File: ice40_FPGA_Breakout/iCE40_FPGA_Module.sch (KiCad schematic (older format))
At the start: 104 parts, among them U1 iCE40HX8_CT256

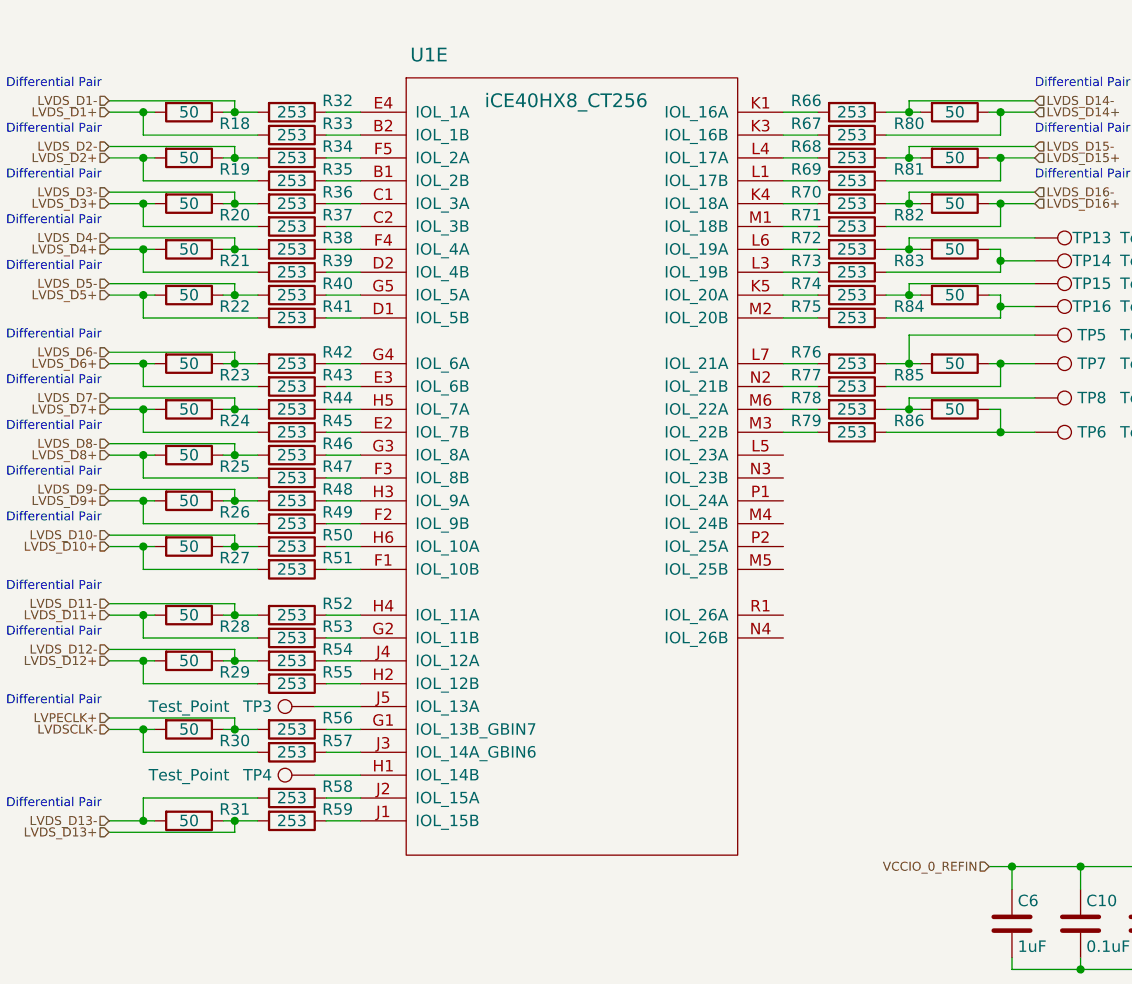
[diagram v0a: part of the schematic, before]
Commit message: Regrouping con't
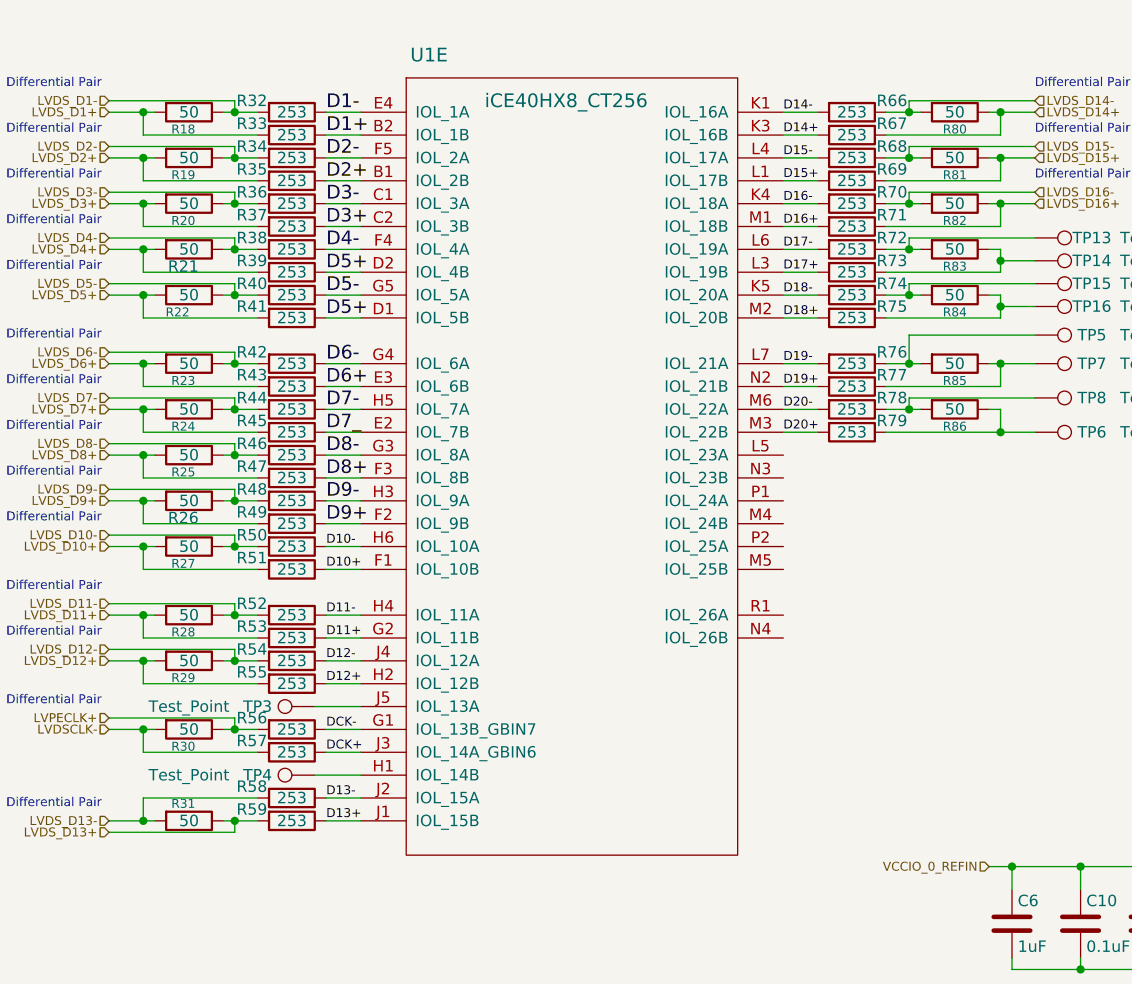
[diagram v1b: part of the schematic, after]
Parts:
- TP1: footprint TestPoint:TestPoint_Plated_Hole_D2.0mm -> TestPoint:TestPoint_THTPad_D1.0mm_Drill0.5mm
- TP2, TP3, TP4: footprint TestPoint:TestPoint_Pad_D2.0mm -> TestPoint:TestPoint_THTPad_D1.0mm_Drill0.5mm
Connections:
- net D2+: now reaches R35.1, U1.B1 (IOL_2B)
- net D1+: now reaches R33.1, U1.B2 (IOL_1B)
- net D3-: now reaches R36.1, U1.C1 (IOL_3A)
- net D3+: now reaches R37.1, U1.C2 (IOL_3B)
- net D5+: now reaches R41.1, U1.D1 (IOL_5B)
- net D5+: now also R39.1, U1.D2 (IOL_4B)
- net D7_: now reaches R45.1, U1.E2 (IOL_7B)
- net D6+: now reaches R43.1, U1.E3 (IOL_6B)
- net D1-: now reaches R32.1, U1.E4 (IOL_1A)
- net D10+: now reaches R51.1, U1.F1 (IOL_10B)
- net D9+: now reaches R49.1, U1.F2 (IOL_9B)
- net D8+: now reaches R47.1, U1.F3 (IOL_8B)
- net D4-: now reaches R38.1, U1.F4 (IOL_4A)
- net D2-: now reaches R34.1, U1.F5 (IOL_2A)
- net DCK-: now reaches R56.1, U1.G1 (IOL_13B_GBIN7)
- net D11+: now reaches R53.1, U1.G2 (IOL_11B)
- net D8-: now reaches R46.1, U1.G3 (IOL_8A)
- net D6-: now reaches R42.1, U1.G4 (IOL_6A)
- net D5-: now reaches R40.1, U1.G5 (IOL_5A)
- net D12+: now reaches R55.1, U1.H2 (IOL_12B)
- net D9-: now reaches R48.1, U1.H3 (IOL_9A)
- net D11-: now reaches R52.1, U1.H4 (IOL_11A)
- net D7-: now reaches R44.1, U1.H5 (IOL_7A)
- net D10-: now reaches R50.1, U1.H6 (IOL_10A)
- net D13+: now reaches R59.1, U1.J1 (IOL_15B)
- net D13-: now reaches R58.1, U1.J2 (IOL_15A)
- net DCK+: now reaches R57.1, U1.J3 (IOL_14A_GBIN6)
- net D12-: now reaches R54.1, U1.J4 (IOL_12A)
- net D14-: now reaches R66.2, U1.K1 (IOL_16A)
- net D14+: now reaches R67.2, U1.K3 (IOL_16B)
- net D16-: now reaches R70.2, U1.K4 (IOL_18A)
- net D18-: now reaches R74.2, U1.K5 (IOL_20A)
- net D15+: now reaches R69.2, U1.L1 (IOL_17B)
- net D17+: now reaches R73.2, U1.L3 (IOL_19B)
- net D15-: now reaches R68.2, U1.L4 (IOL_17A)
- net D17-: now reaches R72.2, U1.L6 (IOL_19A)
- net D19-: now reaches R76.2, U1.L7 (IOL_21A)
- net D16+: now reaches R71.2, U1.M1 (IOL_18B)
- net D18+: now reaches R75.2, U1.M2 (IOL_20B)
- net D20+: now reaches R79.2, U1.M3 (IOL_22B)
- net D20-: now reaches R78.2, U1.M6 (IOL_22A)
- net D19+: now reaches R77.2, U1.N2 (IOL_21B)
